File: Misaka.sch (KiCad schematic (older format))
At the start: 7 parts, among them J1 Battery, SW1 SW_DIP_x03, U2 ATmega2560-16AU, Y1 CSTLS16M0X51-B0

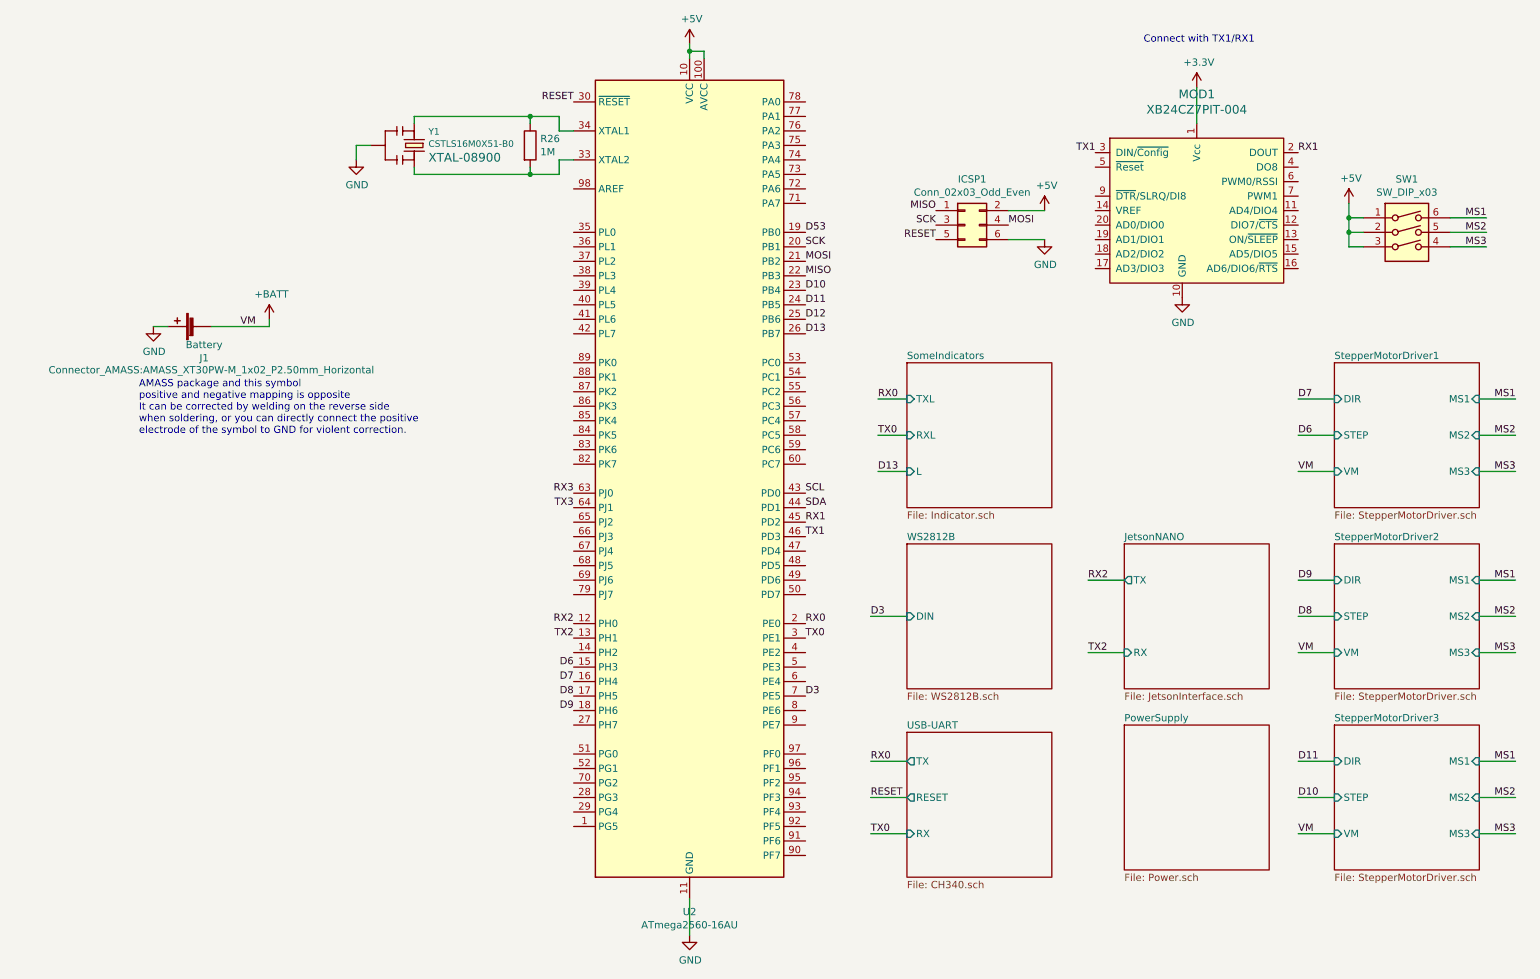
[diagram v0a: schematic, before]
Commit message: DEL LED MS123
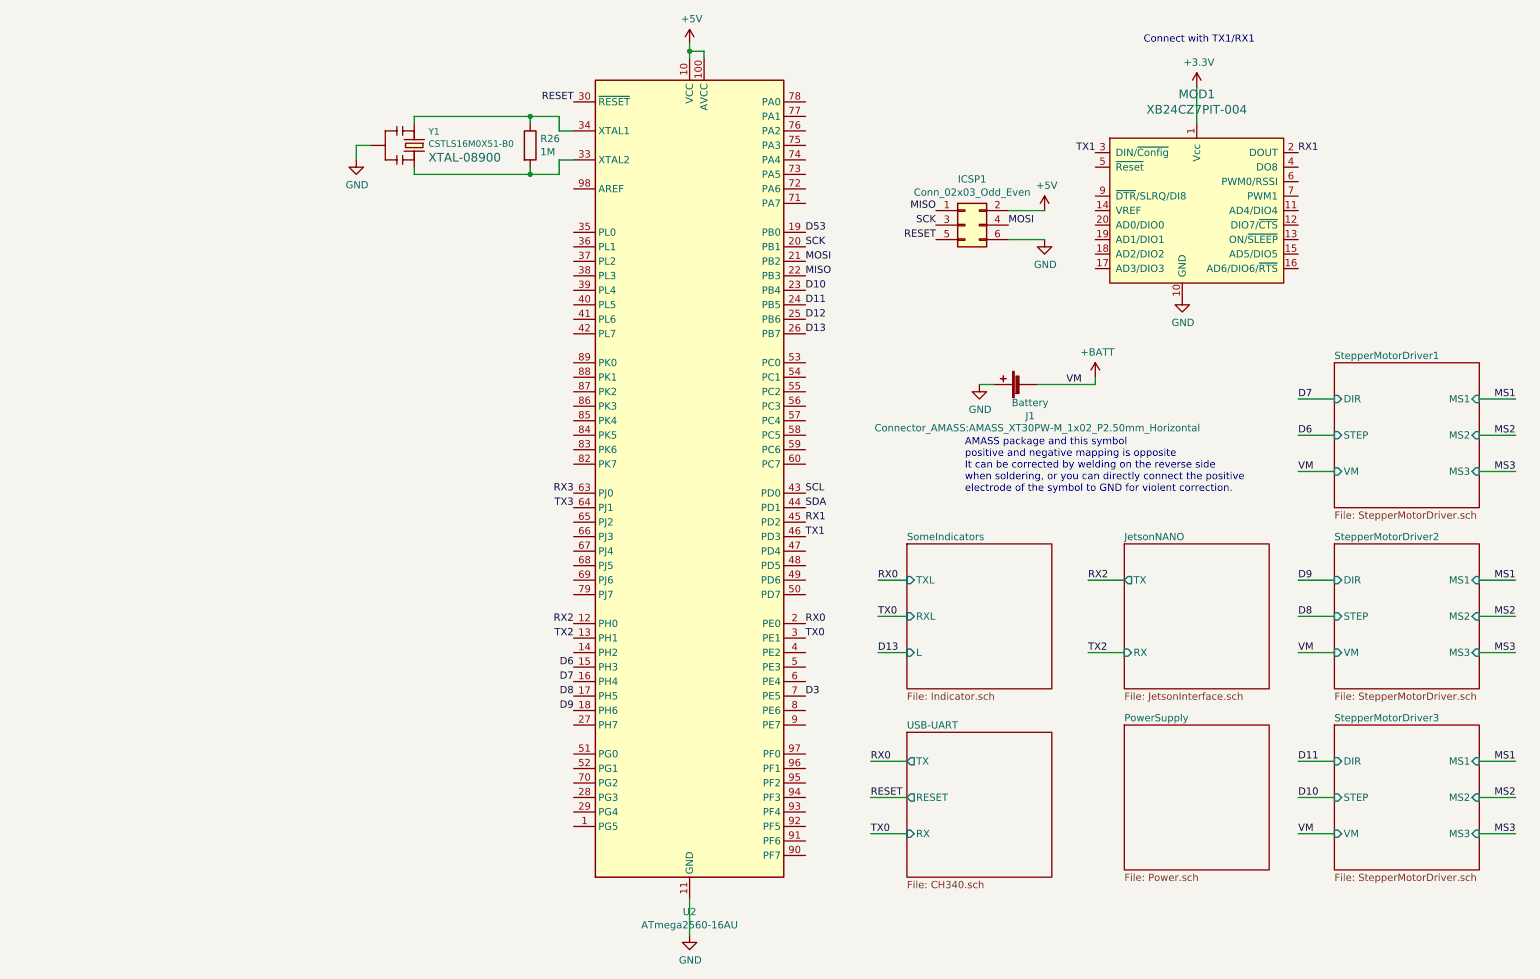
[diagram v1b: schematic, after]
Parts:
- removed SW1: SW_DIP_x03, Button_Switch_SMD:SW_DIP_SPSTx03_Slide_6.7x9.18mm_W8.61mm_P2.54mm_LowProfile, symbol Switch:SW_DIP_x03
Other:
- moved on the sheet: J1
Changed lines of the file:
@@
 $Descr A4 11693 8268
 encoding utf-8
-Sheet 1 9
+Sheet 1 8
 Title ""
 Date ""
@@
 MS3
 $Comp
-L Switch:SW_DIP_x03 SW1
-U 1 1 5E63CD4E
-P 9950 2100
-F 0 "SW1" H 9950 2567 50  0000 C CNN
-F 1 "SW_DIP_x03" H 9950 2476 50  0000 C CNN
-F 2 "Button_Switch_SMD:SW_DIP_SPSTx03_Slide_6.7x9.18mm_W8.61mm_P2.54mm_LowProfile" H 9950 2100 50  0001 C CNN
-F 3 "~" H 9950 2100 50  0001 C CNN
-	1    9950 2100
-	1    0    0    -1
-$EndComp
-$Comp
-L power:+5V #PWR0113
-U 1 1 5E63F269
-P 9550 1800
-F 0 "#PWR0113" H 9550 1650 50  0001 C CNN
-F 1 "+5V" H 9565 1973 50  0000 C CNN
-F 2 "" H 9550 1800 50  0001 C CNN
-F 3 "" H 9550 1800 50  0001 C CNN
-	1    9550 1800
-	1    0    0    -1
-$EndComp
-Wire Wire Line
-	9550 1800 9550 1900
-Wire Wire Line
-	9550 1900 9650 1900
-Wire Wire Line
-	9550 1900 9550 2000
-Wire Wire Line
-	9550 2000 9650 2000
-Connection ~ 9550 1900
-Wire Wire Line
-	9550 2000 9550 2100
-Wire Wire Line
-	9550 2100 9650 2100
-Connection ~ 9550 2000
-Wire Wire Line
-	10250 1900 10500 1900
-Wire Wire Line
-	10250 2000 10500 2000
-Wire Wire Line
-	10250 2100 10500 2100
-Text Label 10500 1900 2    50   ~ 0
-MS1
-Text Label 10500 2000 2    50   ~ 0
-MS2
-Text Label 10500 2100 2    50   ~ 0
-MS3
-$Comp
 L power:GND #PWR0127
 U 1 1 5E64EFCB
@@
 Text Label 5800 3900 0    50   ~ 0
 SDA
-$Sheet
-S 6500 4150 1000 1000
-U 5E6D783B
-F0 "WS2812B" 50
-F1 "WS2812B.sch" 50
-F2 "DIN" I L 6500 4650 50
-$EndSheet
 Text Label 5800 5200 0    50   ~ 0
 D3
-Wire Wire Line
-	6500 4650 6250 4650
-Text Label 6250 4650 0    50   ~ 0
-D3
-$Sheet
-S 6500 2900 1000 1000
+$Sheet
+S 6500 4150 1000 1000
 U 5E76060A
 F0 "SomeIndicators" 50
 F1 "Indicator.sch" 50
-F2 "TXL" I L 6500 3150 50
-F3 "RXL" I L 6500 3400 50
-F4 "L" I L 6500 3650 50
-$EndSheet
-Wire Wire Line
-	6500 3150 6300 3150
-Wire Wire Line
-	6500 3400 6300 3400
-Wire Wire Line
-	6500 3650 6300 3650
-Text Label 6300 3400 0    50   ~ 0
+F2 "TXL" I L 6500 4400 50
+F3 "RXL" I L 6500 4650 50
+F4 "L" I L 6500 4900 50
+$EndSheet
+Wire Wire Line
+	6500 4400 6300 4400
+Wire Wire Line
+	6500 4650 6300 4650
+Wire Wire Line
+	6500 4900 6300 4900
+Text Label 6300 4650 0    50   ~ 0
 TX0
-Text Label 6300 3150 0    50   ~ 0
+Text Label 6300 4400 0    50   ~ 0
 RX0
-Text Label 6300 3650 0    50   ~ 0
+Text Label 6300 4900 0    50   ~ 0
 D13
 Text Label 7800 1450 2    50   ~ 0
@@
 $EndSheet
 Wire Wire Line
-	1700 2650 2100 2650
+	7400 3050 7800 3050
 $Comp
 L power:GND #PWR0117
 U 1 1 5E622AF8
-P 1300 2650
-F 0 "#PWR0117" H 1300 2400 50  0001 C CNN
-F 1 "GND" H 1305 2477 50  0000 C CNN
-F 2 "" H 1300 2650 50  0001 C CNN
-F 3 "" H 1300 2650 50  0001 C CNN
-	1    1300 2650
-	1    0    0    -1
-$EndComp
-Text Label 1900 2650 0    50   ~ 0
+P 7000 3050
+F 0 "#PWR0117" H 7000 2800 50  0001 C CNN
+F 1 "GND" H 7005 2877 50  0000 C CNN
+F 2 "" H 7000 3050 50  0001 C CNN
+F 3 "" H 7000 3050 50  0001 C CNN
+	1    7000 3050
+	1    0    0    -1
+$EndComp
+Text Label 7600 3050 0    50   ~ 0
 VM
 Wire Wire Line
-	2100 2650 2100 2600
+	7800 3050 7800 3000
 $Comp
 L power:+BATT #PWR0152
 U 1 1 5E62480E
-P 2100 2600
-F 0 "#PWR0152" H 2100 2450 50  0001 C CNN
-F 1 "+BATT" H 2115 2773 50  0000 C CNN
-F 2 "" H 2100 2600 50  0001 C CNN
-F 3 "" H 2100 2600 50  0001 C CNN
-	1    2100 2600
+P 7800 3000
+F 0 "#PWR0152" H 7800 2850 50  0001 C CNN
+F 1 "+BATT" H 7815 3173 50  0000 C CNN
+F 2 "" H 7800 3000 50  0001 C CNN
+F 3 "" H 7800 3000 50  0001 C CNN
+	1    7800 3000
 	1    0    0    -1
 $EndComp
 Text Label 9200 1450 0    50   ~ 0
 RX1
-Text Notes 1200 3400 0    50   ~ 0
+Text Notes 6900 3800 0    50   ~ 0
 AMASS package and this symbol \npositive and negative mapping is opposite\nIt can be corrected by welding on the reverse side\nwhen soldering, or you can directly connect the positive \nelectrode of the symbol to GND for violent correction.
 $Comp
 L Device:Battery_Cell J1
 U 1 1 5E620D8E
-P 1600 2650
-F 0 "J1" V 1383 2600 50  0000 C CNN
-F 1 "Battery" V 1474 2600 50  0000 C CNN
-F 2 "Connector_AMASS:AMASS_XT30PW-M_1x02_P2.50mm_Horizontal" V 1300 2550 50  0000 C CNN
-F 3 "~" H 1600 2600 50  0001 C CNN
-	1    1600 2650
+P 7300 3050
+F 0 "J1" V 7083 3000 50  0000 C CNN
+F 1 "Battery" V 7174 3000 50  0000 C CNN
+F 2 "Connector_AMASS:AMASS_XT30PW-M_1x02_P2.50mm_Horizontal" V 7000 2950 50  0000 C CNN
+F 3 "~" H 7300 3000 50  0001 C CNN
+	1    7300 3050
 	0    -1   -1   0
 $EndComp
 Wire Wire Line
-	1300 2650 1400 2650
+	7000 3050 7100 3050
 $EndSCHEMATC
